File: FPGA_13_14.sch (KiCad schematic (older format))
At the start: 15 parts, among them SW1 SW_DIP_x01, U1 XC7A100T-2FGG484C, U11 SN74LVC1G125DCKT, U30 S25FL128SAGMFIR01

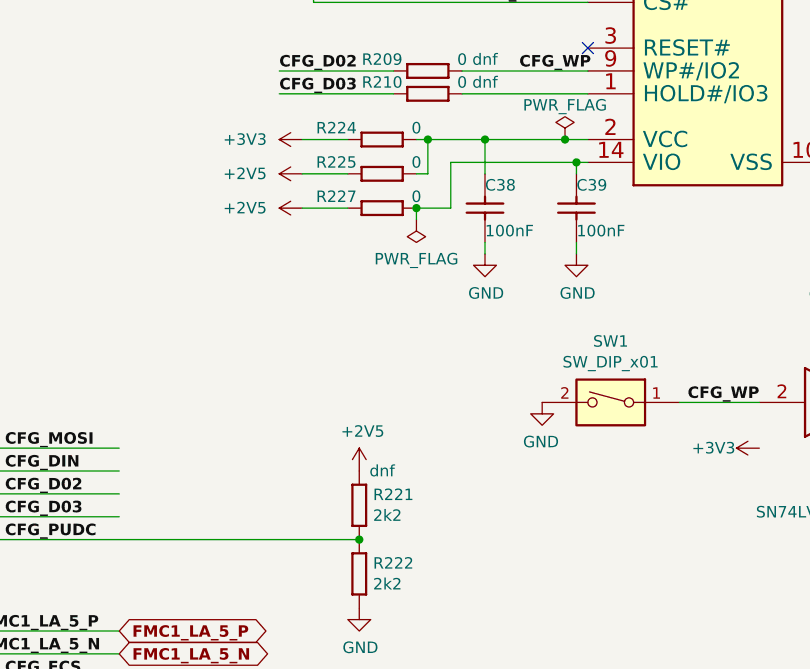
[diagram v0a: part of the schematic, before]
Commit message: applied all required amendments to the project
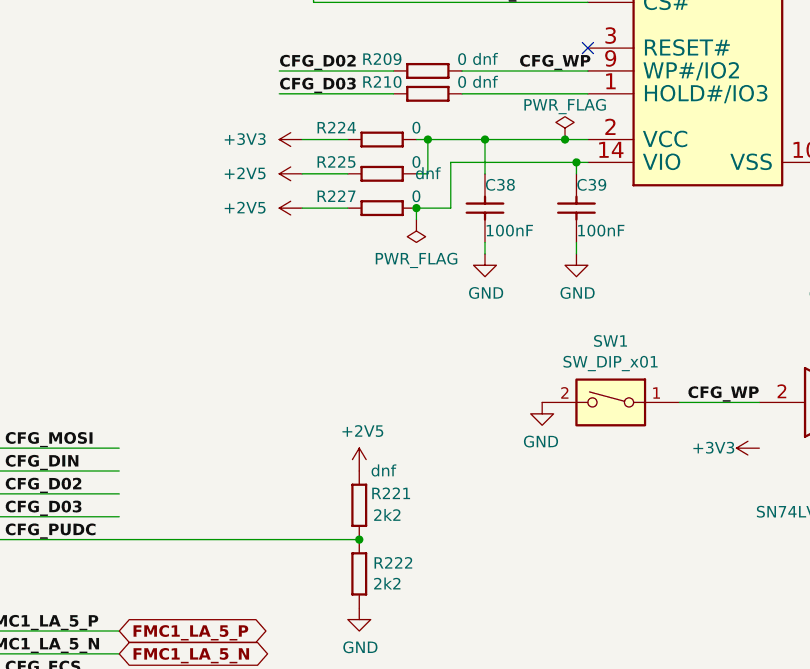
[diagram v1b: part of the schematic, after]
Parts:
- R225: config (none) -> dnf
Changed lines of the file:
@@
 EESchema Schematic File Version 4
 LIBS:AMC_FMC_Carrier-PcbDoc-cache
-EELAYER 29 0
+EELAYER 30 0
 EELAYER END
 $Descr A3 16535 11693
@@
 AR Path="/5C907554/5CAAC367/5F9465E2" Ref="R?"  Part="1"
 AR Path="/5C907554/5CC8CB69/5F9465E2" Ref="R221"  Part="1"
-F 0 "R221" V 12304 3360 50  0000 L CNN
+F 0 "R221" V 12300 3350 50  0000 L CNN
 F 1 "R0402_2K2_1%_0.0625W_100PPM" H 12200 3090 60  0001 L CNN
 F 2 "RESC1005X40N" H 12200 2280 60  0001 L CNN
@@
 F 40 "Resistors SMD" H 12200 -420 60  0001 L CNN "Library Name"
 F 41 "This work is licensed under the Creative Commons CC-BY-SA 4.0 License. To the extent that circuit schematics that use Licensed Material can be considered to be ‘Adapted Material’, then the copyright holder waives article 3.b of the license with respect to these schematics." H 12200 -510 60  0001 L CNN "License"
-F 42 "dnf" V 12200 3400 50  0000 C CNN "config"
+F 42 "dnf" V 12200 3350 50  0000 L CNN "config"
 	1    12200 3300
 	0    1    1    0
@@
 F 40 "Resistors SMD" H 12150 -1720 60  0001 L CNN "Library Name"
 F 41 "This work is licensed under the Creative Commons CC-BY-SA 4.0 License. To the extent that circuit schematics that use Licensed Material can be considered to be ‘Adapted Material’, then the copyright holder waives article 3.b of the license with respect to these schematics." H 12150 -1810 60  0001 L CNN "License"
+F 42 "dnf" H 12500 2000 50  0000 C CNN "config"
 	1    12150 2000
 	1    0    0    -1
